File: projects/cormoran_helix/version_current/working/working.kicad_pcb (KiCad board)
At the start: 2 copper layers, 132 x 94 mm, 223 parts, among them J1 MJ-4PP-9, P1 CONN_01X01, P2 CONN_01X01, P3 OLED, P4 LED, P5 ICSP, SW1 SW_PUSH, SW10 SW_PUSH, SW11 SW_PUSH, SW12 SW_PUSH, SW13 SW_PUSH, SW14 SW_PUSH, SW15 SW_PUSH, SW16 SW_PUSH, SW17 SW_PUSH, SW18 SW_PUSH, SW19 SW_PUSH, SW2 SW_PUSH, SW20 SW_PUSH, SW21 SW_PUSH, SW22 SW_PUSH, SW23 SW_PUSH, SW24 SW_PUSH, SW25 SW_PUSH, SW26 SW_PUSH, SW27 SW_PUSH, SW28 SW_PUSH, SW29 SW_PUSH, SW3 SW_PUSH, SW30 SW_PUSH, SW31 SW_PUSH, SW32 SW_PUSH, SW33 Reset, SW4 SW_PUSH, SW5 SW_PUSH, SW6 SW_PUSH, SW7 SW_PUSH, SW8 SW_PUSH, SW9 SW_PUSH, U1 ProMicro, U10 SK6812mini, U11 SK6812mini, U12 SK6812mini, U13 SK6812mini, U14 SK6812mini, U15 SK6812mini, U16 SK6812mini, U17 SK6812mini, U18 SK6812mini, U19 SK6812mini, U2 SK6812mini, U20 SK6812mini, U21 SK6812mini, U22 SK6812mini, U23 SK6812mini, U24 SK6812mini, U25 SK6812mini, U26 SK6812mini, U27 SK6812mini, U28 SK6812mini, U29 SK6812mini, U3 SK6812mini, U30 SK6812mini, U31 SK6812mini, U32 SK6812mini, U33 SK6812mini, U4 SK6812mini, U5 SK6812mini, U6 SK6812mini, U7 SK6812mini, U8 SK6812mini, U9 SK6812mini

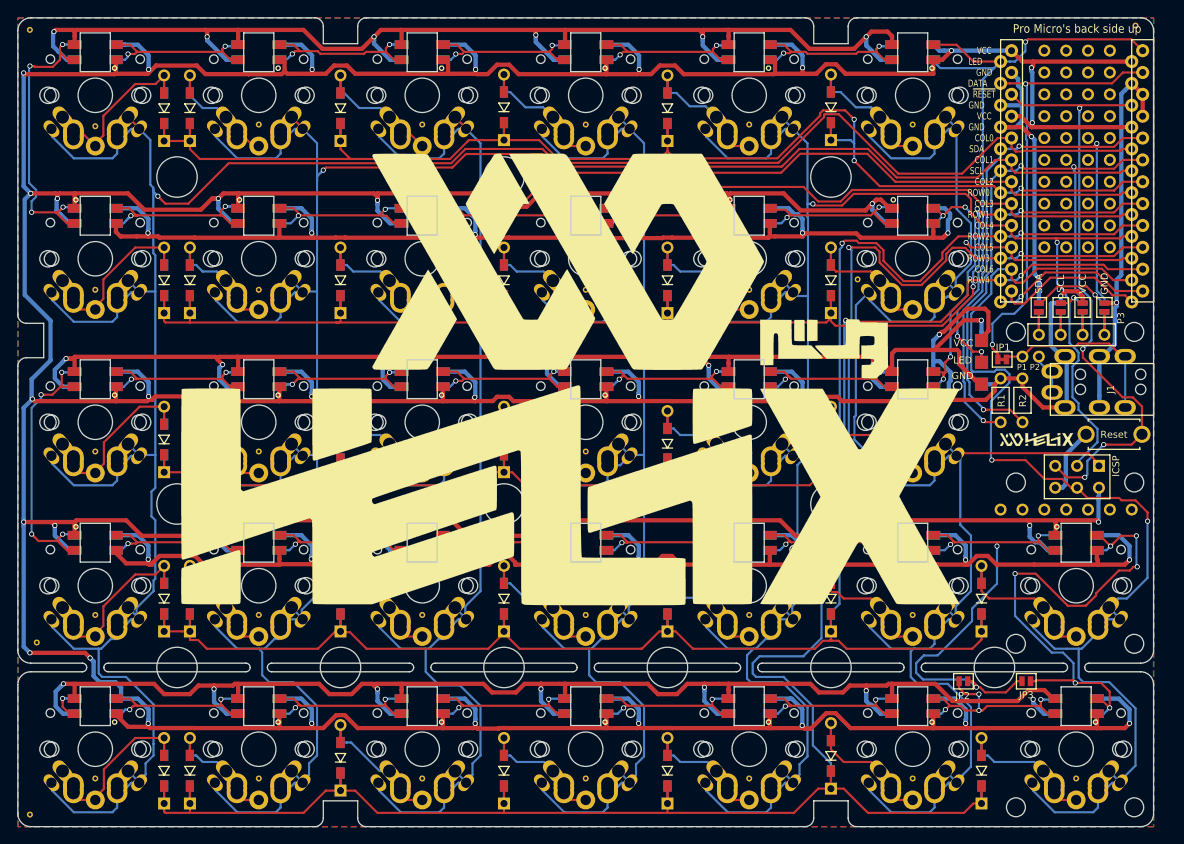
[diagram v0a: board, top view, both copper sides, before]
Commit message: some generations
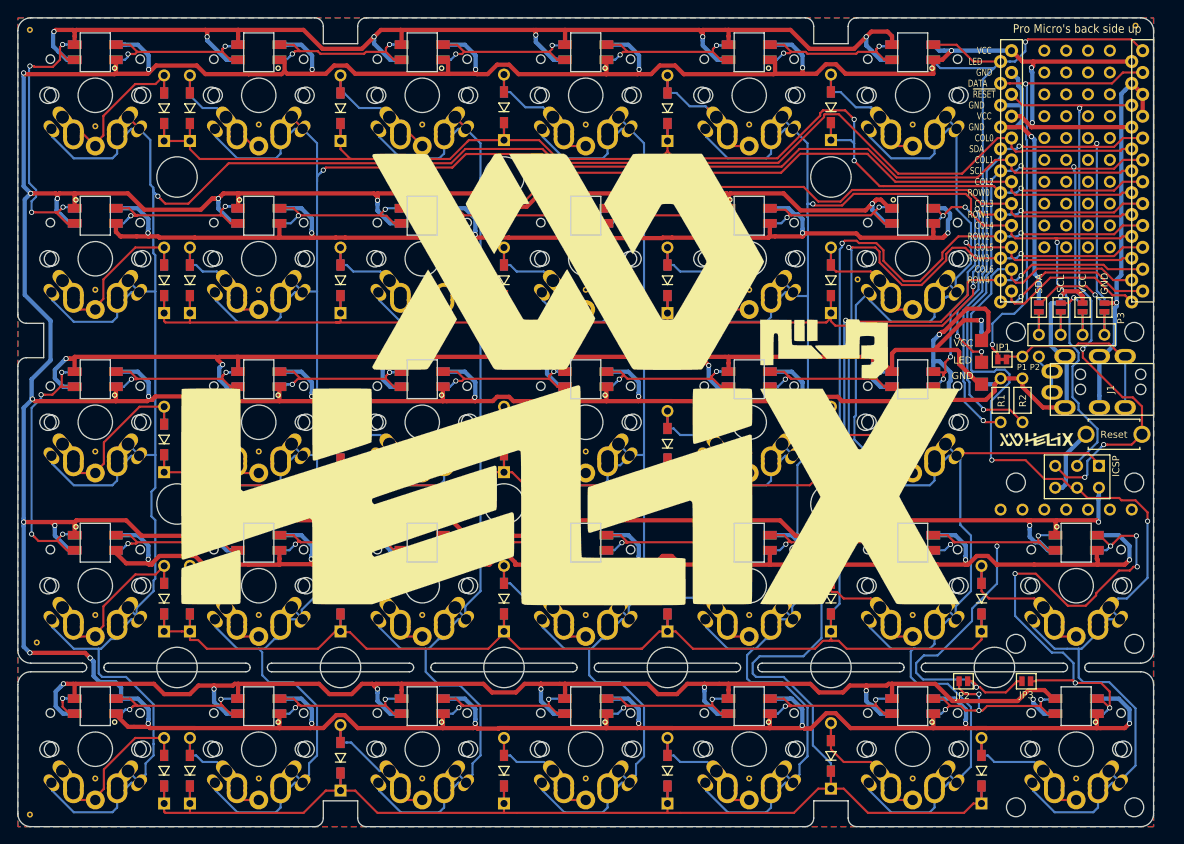
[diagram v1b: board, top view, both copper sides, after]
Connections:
- net /~RESET renamed /~{RESET}
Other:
- net class Default removed
- net class bold removed
- board text added: "~{RESET}"
- board text removed: "~RESET"

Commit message: updated all projects from src
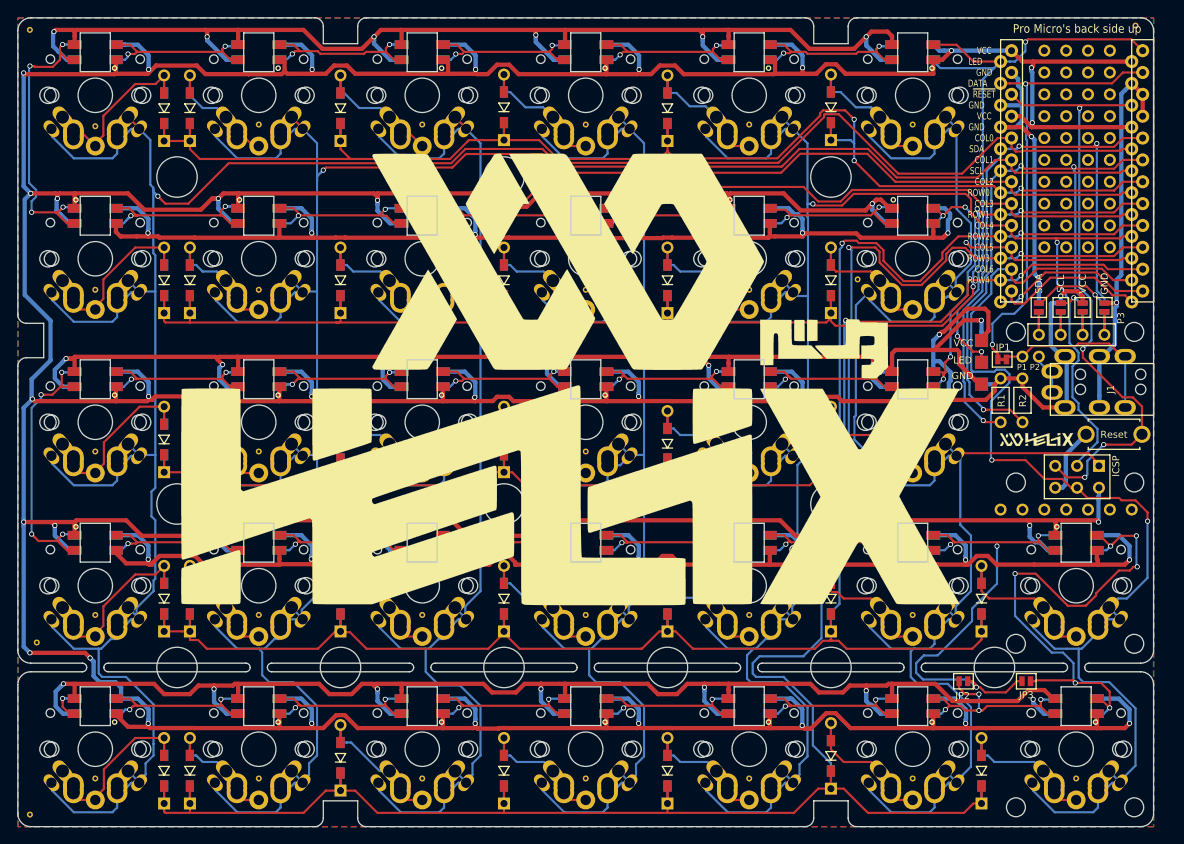
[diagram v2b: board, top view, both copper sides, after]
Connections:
- net /~{RESET} renamed /~RESET
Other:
- net class Default added: clearance 0.2, trace_width 0.25, via_dia 0.6, via_drill 0.4
- net class bold added: clearance 0.2, trace_width 0.5, via_dia 0.6, via_drill 0.4
- board text added: "~RESET"
- board text removed: "~{RESET}"
